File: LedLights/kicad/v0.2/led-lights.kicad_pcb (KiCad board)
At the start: 2 copper layers, 82.6 x 71.1 mm, 15 parts, among them P1 Power input, P2 PIR1 connector, P3 LDR connector, P5 LED 1, P6 LED 2, P7 PIR2 connector, P8 LED 3, P9 HC-05 connector, U1 arduino_nano

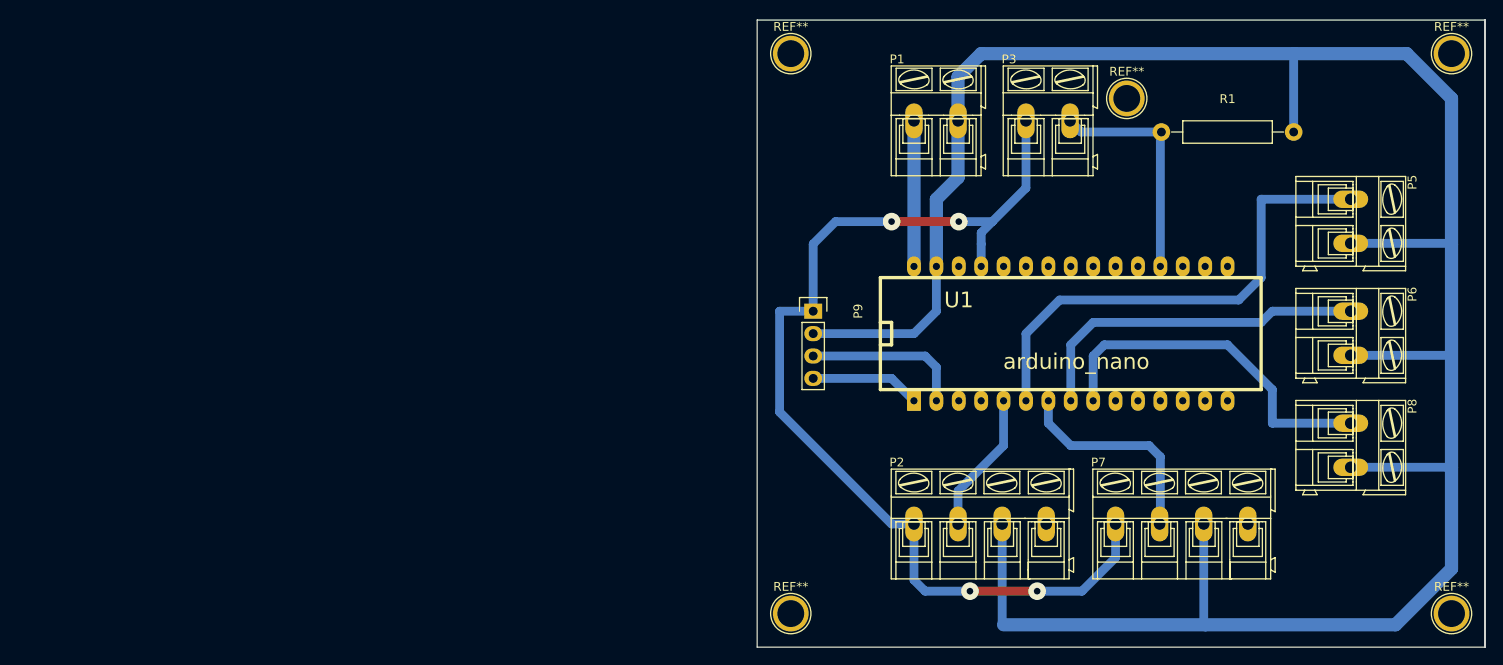
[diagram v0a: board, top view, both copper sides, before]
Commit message: Kicad and stuff
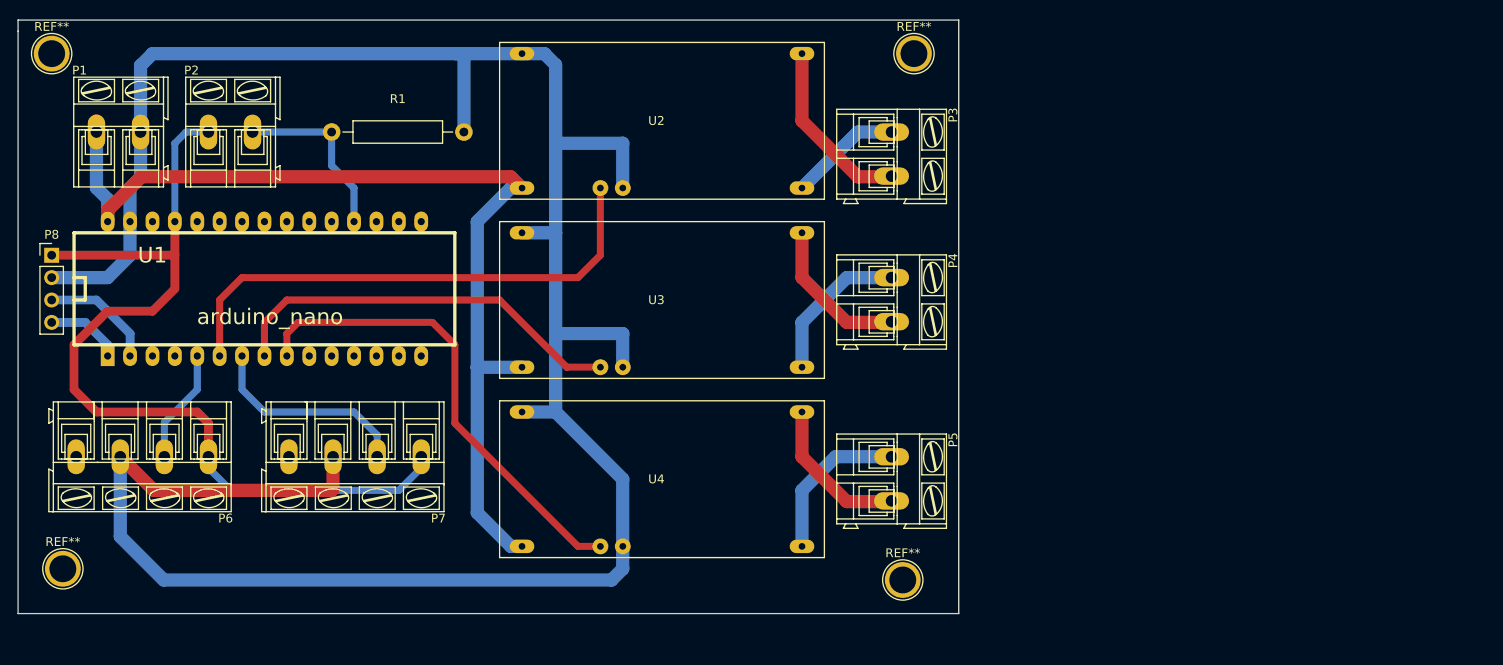
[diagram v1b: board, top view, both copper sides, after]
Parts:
- removed P9: HC-05 connector, Socket_Strips:Socket_Strip_Straight_1x04
- removed the REF** at (105.4, 62.2)
- removed the REF** at (180.3, 62.2)
- removed the REF** at (180.3, 125.7)
- removed the REF** at (105.4, 125.7)
- removed the REF** at (143.5, 67.3)
- added P4: LED 2, Connectors:AK300-2, F.Cu at (116.8, 87.6)
- added REF**: 1pin, Connectors:1pin, F.Cu at (119.4, 62.2)
- added REF**: 1pin, Connectors:1pin, F.Cu at (118.1, 121.9)
- added REF**: 1pin, Connectors:1pin, F.Cu at (22.9, 120.7)
- added REF**: 1pin, Connectors:1pin, F.Cu at (21.6, 62.2)
- added U2: LED_Driver_700mA, lib:LED_Driver_700mA_foot, F.Cu at (90.2, 69.8)
- added U3: LED_Driver_700mA, lib:LED_Driver_700mA_foot, F.Cu at (90.2, 90.2)
- added U4: LED_Driver_700mA, lib:LED_Driver_700mA_foot, F.Cu at (90.2, 110.5)
- P1: footprint Connect:AK300-2 -> Connectors:AK300-2
- P2: value PIR1 connector -> LDR connector; footprint Connect:AK300-4 -> Connectors:AK300-2
- P3: value LDR connector -> LED 1; footprint Connect:AK300-2 -> Connectors:AK300-2
- P5: value LED 1 -> LED 3; footprint Connect:AK300-2 -> Connectors:AK300-2
- P6: value LED 2 -> PIR1 connector; footprint Connect:AK300-2 -> Connectors:AK300-4
- P7: footprint Connect:AK300-4 -> Connectors:AK300-4
- P8: value LED 3 -> HC-05 connector; footprint Connect:AK300-2 -> Socket_Strips:Socket_Strip_Straight_1x04_Pitch2.54mm
- R1: footprint Resistors_ThroughHole:Resistor_Horizontal_RM15mm -> Resistors_General:Resistor_Horizontal_RM15mm
- moved P8 148.5 mm to (21.6, 85.1), turned to 0 degrees
- moved P6 130.6 mm to (39.4, 108.0), turned to 180 degrees
- moved R1 101.6 mm to (53.3, 71.1)
- moved P1 92.7 mm to (26.7, 71.1)
- moved U1 91.6 mm to (47.0, 88.9)
- moved P2 91.5 mm to (39.4, 71.1)
- moved P7 79.1 mm to (63.5, 108.0), turned to 180 degrees
- moved P5 59.7 mm to (116.8, 108.0)
- moved P3 15.3 mm to (116.8, 71.1), turned to 270 degrees
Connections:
- P2 pad 2: pirInPin1 -> Net-(P2-Pad2)
- P3 pad 1: +5V -> Net-(P3-Pad1)
- P5 pad 1: ledPwmPin1 -> Net-(P5-Pad1)
- P5 pad 2: GND -> Net-(P5-Pad2)
- P6 pad 1: ledPwmPin2 -> +5V
- P6 pad 2: GND -> pirInPin1
- P8 pad 1: ledPwmPin3 -> +5V
- R1 pad 1: Net-(P3-Pad2) -> Net-(P2-Pad2)
- U1 pad A0: Net-(P3-Pad2) -> Net-(P2-Pad2)
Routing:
- net +12V: track 16.5 -> 113.7 mm
- net Net-(P2-Pad2): track 0.00 -> 20.2 mm
- net Net-(P5-Pad1): track 0.00 -> 18.1 mm
- net Net-(P5-Pad2): track 0.00 -> 17.4 mm
- net Net-(P4-Pad2): track 0.00 -> 17.4 mm
- net Net-(P4-Pad1): track 0.00 -> 17.3 mm
- net +5V: track 118.5 -> 104.6 mm, vias 4 -> 0
- net ledPwmPin3: track 40.7 -> 54.4 mm
- net Net-(P3-Pad1): track 0.00 -> 12.8 mm
- net ledPwmPin2: track 39.7 -> 46.1 mm
- net Net-(P3-Pad2): track 26.2 -> 20.4 mm
- net RX: track 18.3 -> 13.0 mm
- net GND: track 275.7 -> 280.1 mm
- net TX: track 12.5 -> 8.67 mm
- net ledPwmPin1: track 56.0 -> 59.3 mm
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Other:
- board size 82.6 x 71.1 mm -> 106.7 x 67.3 mm
